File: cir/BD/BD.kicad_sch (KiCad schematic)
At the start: 11 parts, among them J1 Conn_01x06_Socket, J2 Conn_01x04_Socket, J4 Barrel_Jack_MountingPin, SW1 SW_Push, SW2 SW_Push

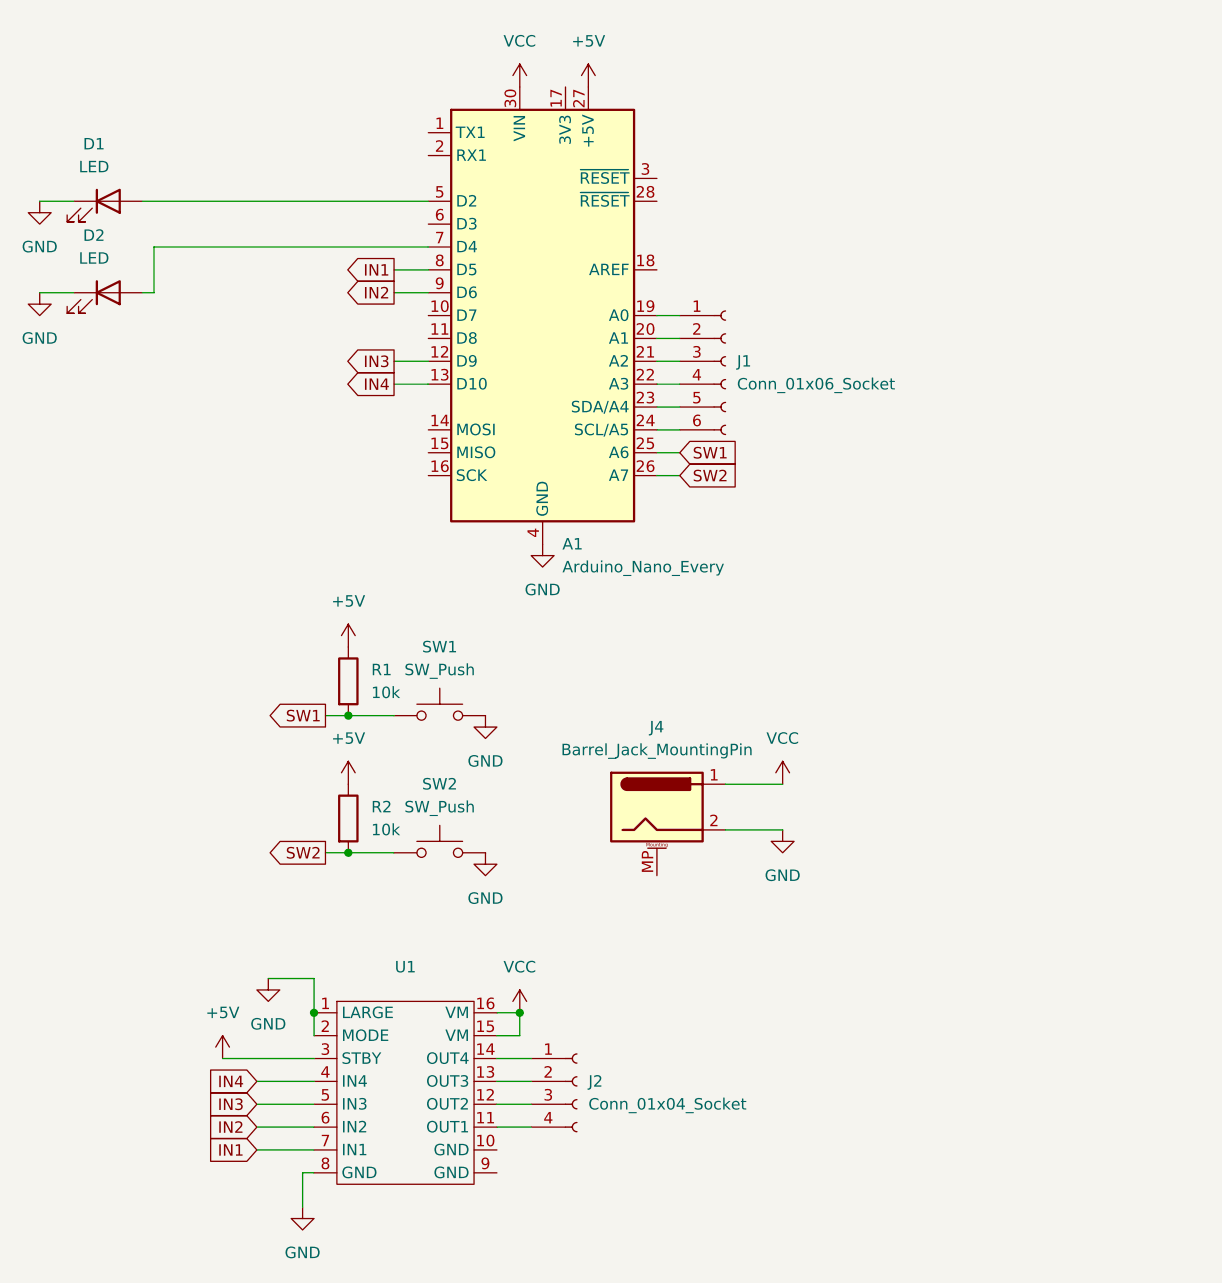
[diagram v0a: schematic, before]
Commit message: up
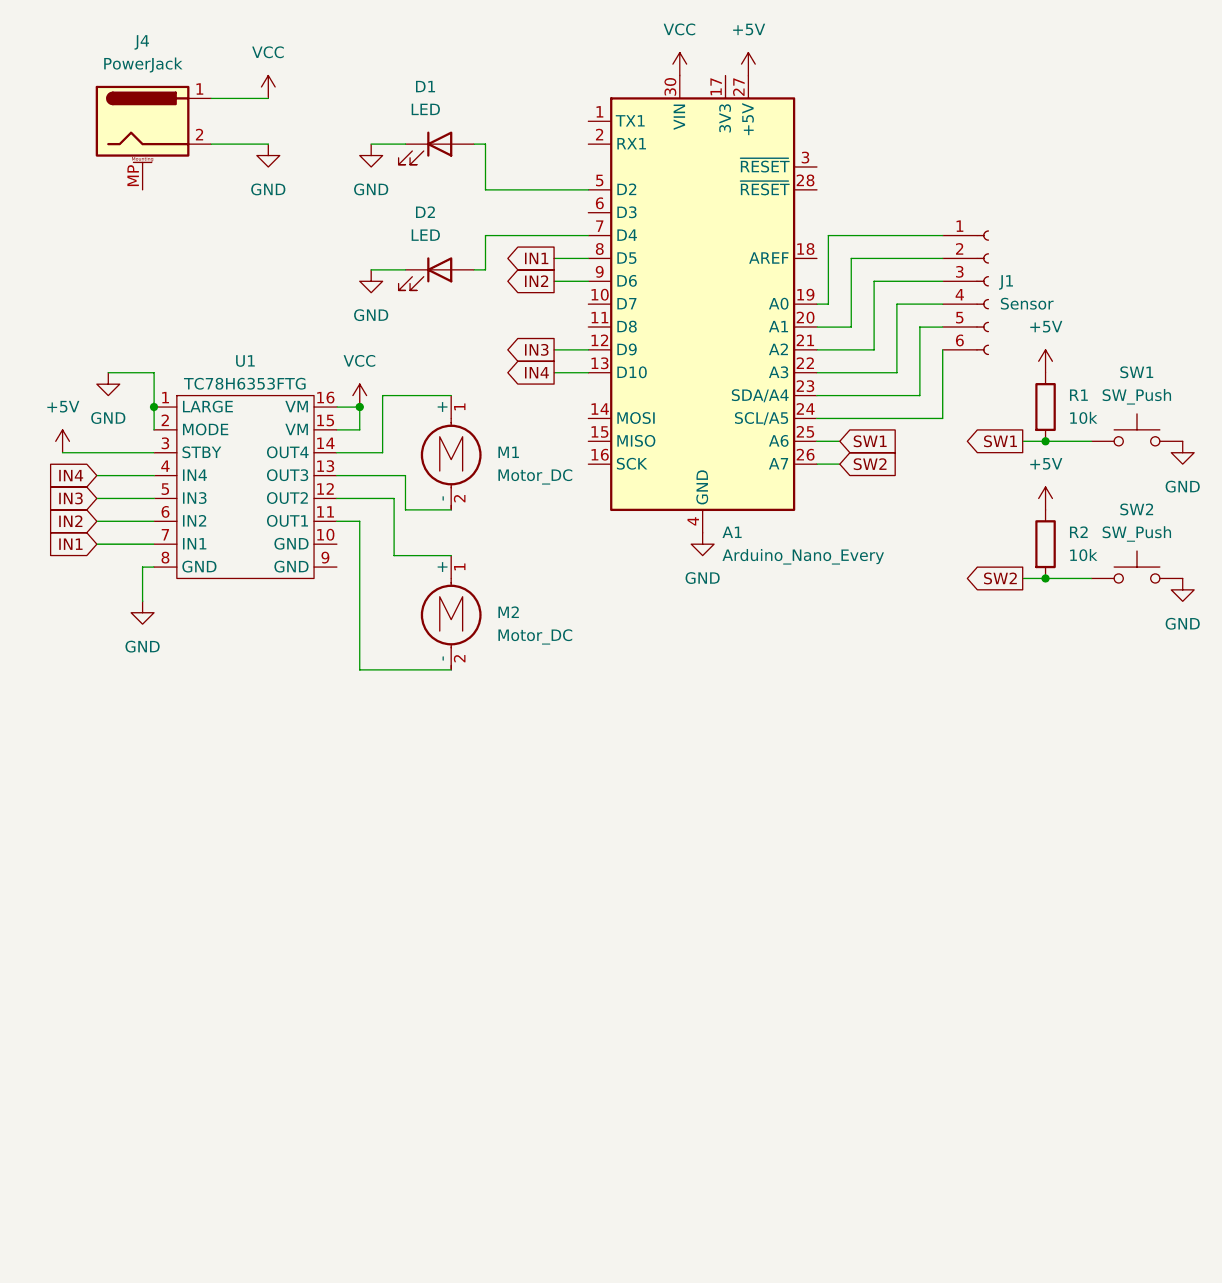
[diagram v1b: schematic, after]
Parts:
- removed J2: Conn_01x04_Socket, Connector_PinSocket_2.54mm:PinSocket_1x04_P2.54mm_Vertical, symbol Connector:Conn_01x04_Socket
- added M1, M2: Motor_DC, symbol Motor:Motor_DC
- J1: value Conn_01x06_Socket -> Sensor
- J4: value Barrel_Jack_MountingPin -> PowerJack
- U1: value ~ -> TC78H6353FTG
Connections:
- net at U1.14 (OUT4): now also M1.1 (+)
- net at U1.13 (OUT3): now also M1.2 (-)
- net at U1.12 (OUT2): now also M2.1 (+)
- net at U1.11 (OUT1): now also M2.2 (-)
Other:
- moved on the sheet: A1, D1, D2, J1, J4, R1, R2, SW1, SW2, U1
